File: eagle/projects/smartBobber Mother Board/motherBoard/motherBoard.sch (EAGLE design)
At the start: 62 parts, among them J1 10118193-0001LF, J6 1053131202, Q1 2A/20V/150mΩ, Q2 MMBT3904, U1 MCP7384XX, U2 MT3608, U3 LTC3531ES6-3_3, Y1 ECS-40-S-4X

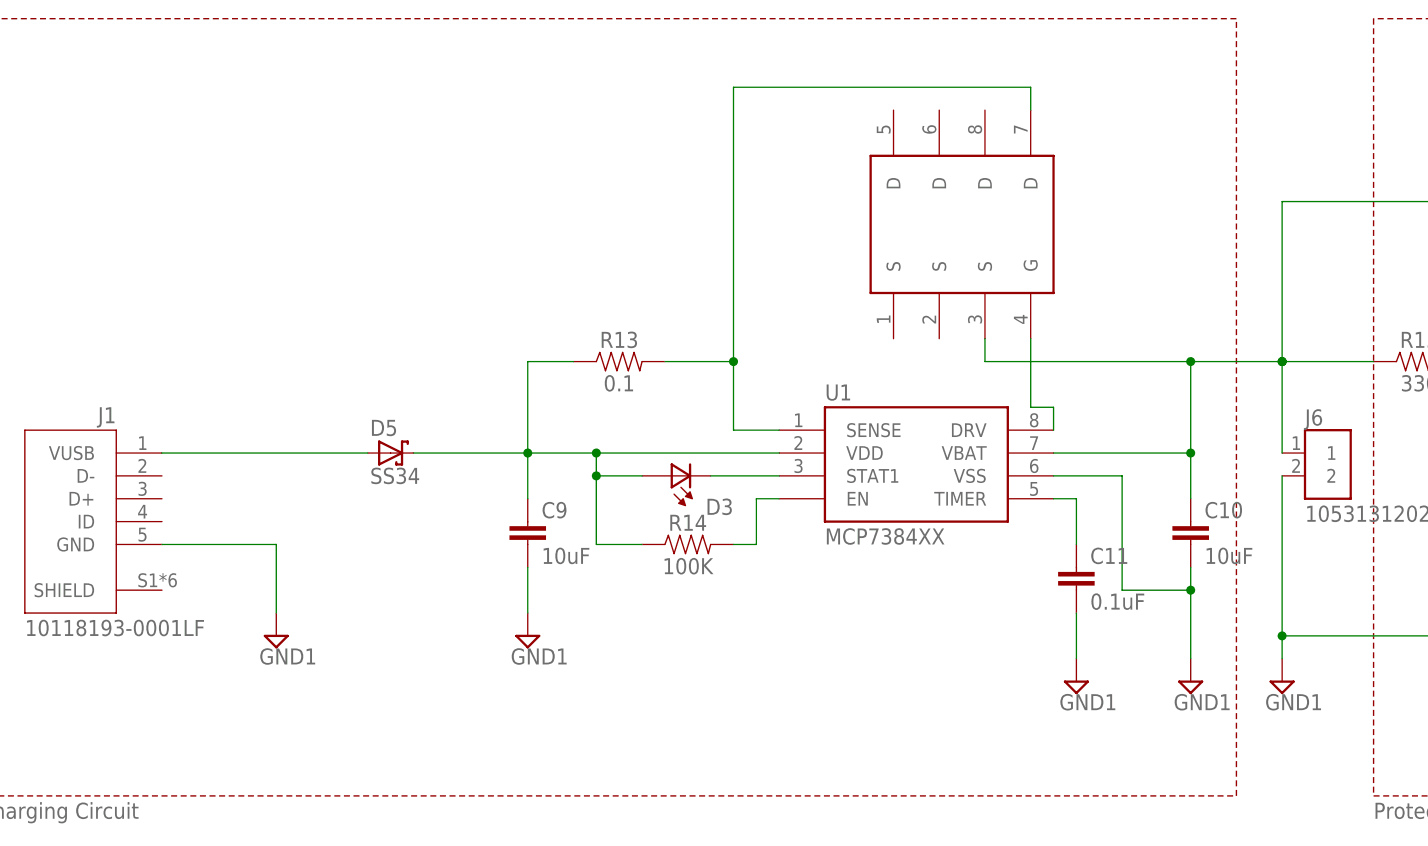
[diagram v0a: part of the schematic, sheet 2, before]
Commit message: MCP73831
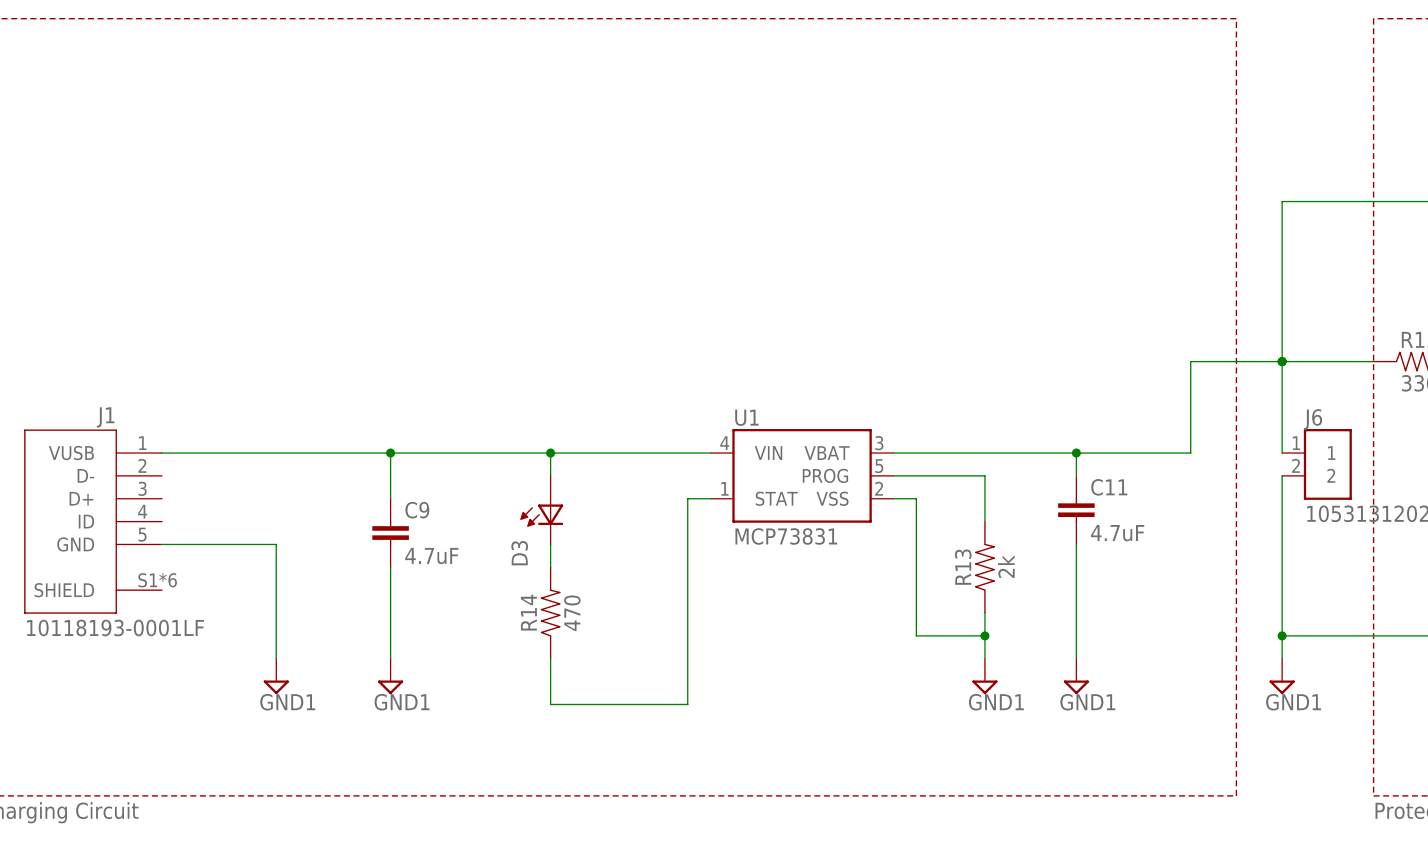
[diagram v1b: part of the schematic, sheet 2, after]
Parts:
- removed C10: 10uF, SparkFun-Capacitors:10UF-0603-6.3V-20%
- removed D5: SS34, SS34:SS34
- removed U$3: NDS8434, NDS8434:NDS8434
- C11: value 0.1uF -> 4.7uF
- C9: value 10uF -> 4.7uF
- R13: value 0.1 -> 2k
- R14: value 100K -> 470
- U1: value MCP7384XX -> MCP73831; device SparkFun-IC-Power:MCP7384XX -> SparkFun-IC-Power:MCP73831
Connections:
- removed net N$10: U$3.G, U1.DRV
- removed net N$17: C11.1, U1.TIMER
- removed net N$19: C10.1, J6.1, R15.1, S1.1, U$3.S@3, U1.VBAT
- net GND: now also R13.1; no longer C10.2
- net N$11: now also C9.1, D3.A2, U1.VIN; no longer D5.A
- net N$2: now also D3.K2, R14.2; no longer C9.1, D3.A2, D5.C, R13.1, R14.1, U1.VDD
- net N$7: now also R14.1, U1.STAT; no longer D3.K2, U1.STAT1
- net N$8: now also C11.1, J6.1, R15.1, S1.1, U1.VBAT; no longer R14.2, U1.EN
- net N$9: now also U1.PROG; no longer U$3.D@1, U1.SENSE
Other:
- moved on the sheet: C11, C9, D3, R13, R14
